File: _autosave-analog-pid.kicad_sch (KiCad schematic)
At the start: 24 parts, among them J1 Conn_01x06_Socket, U1 MCP6004, U2 Opamp_Dual, U3 MCP6004

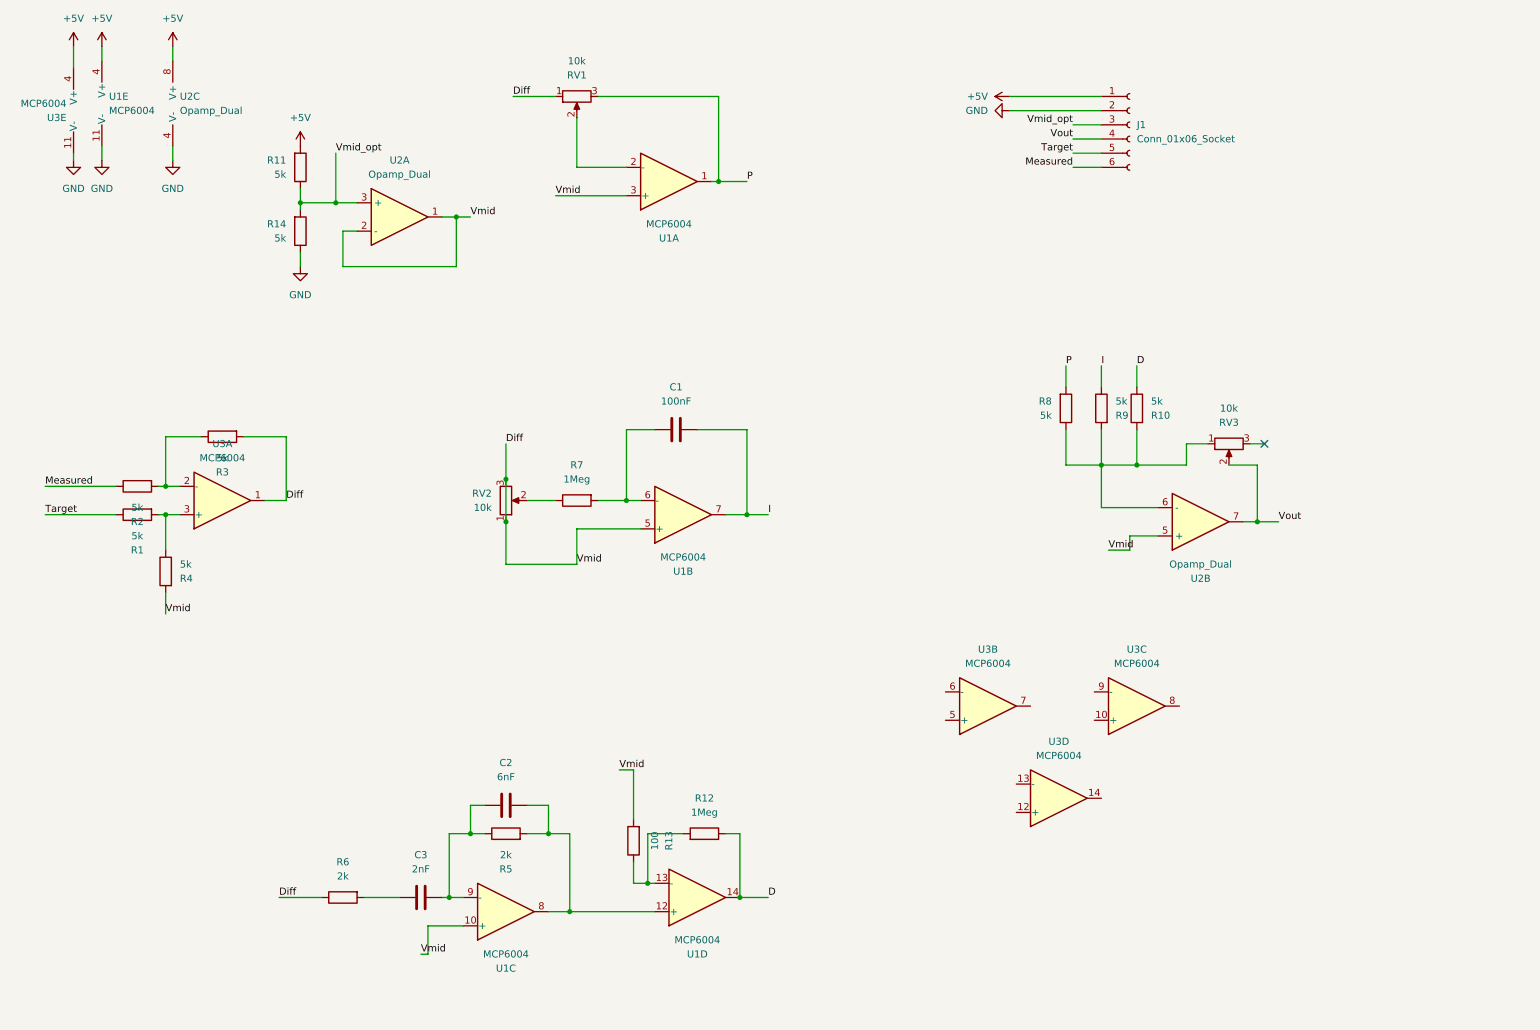
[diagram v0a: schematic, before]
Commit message: second commit before i add even  more fking stuff
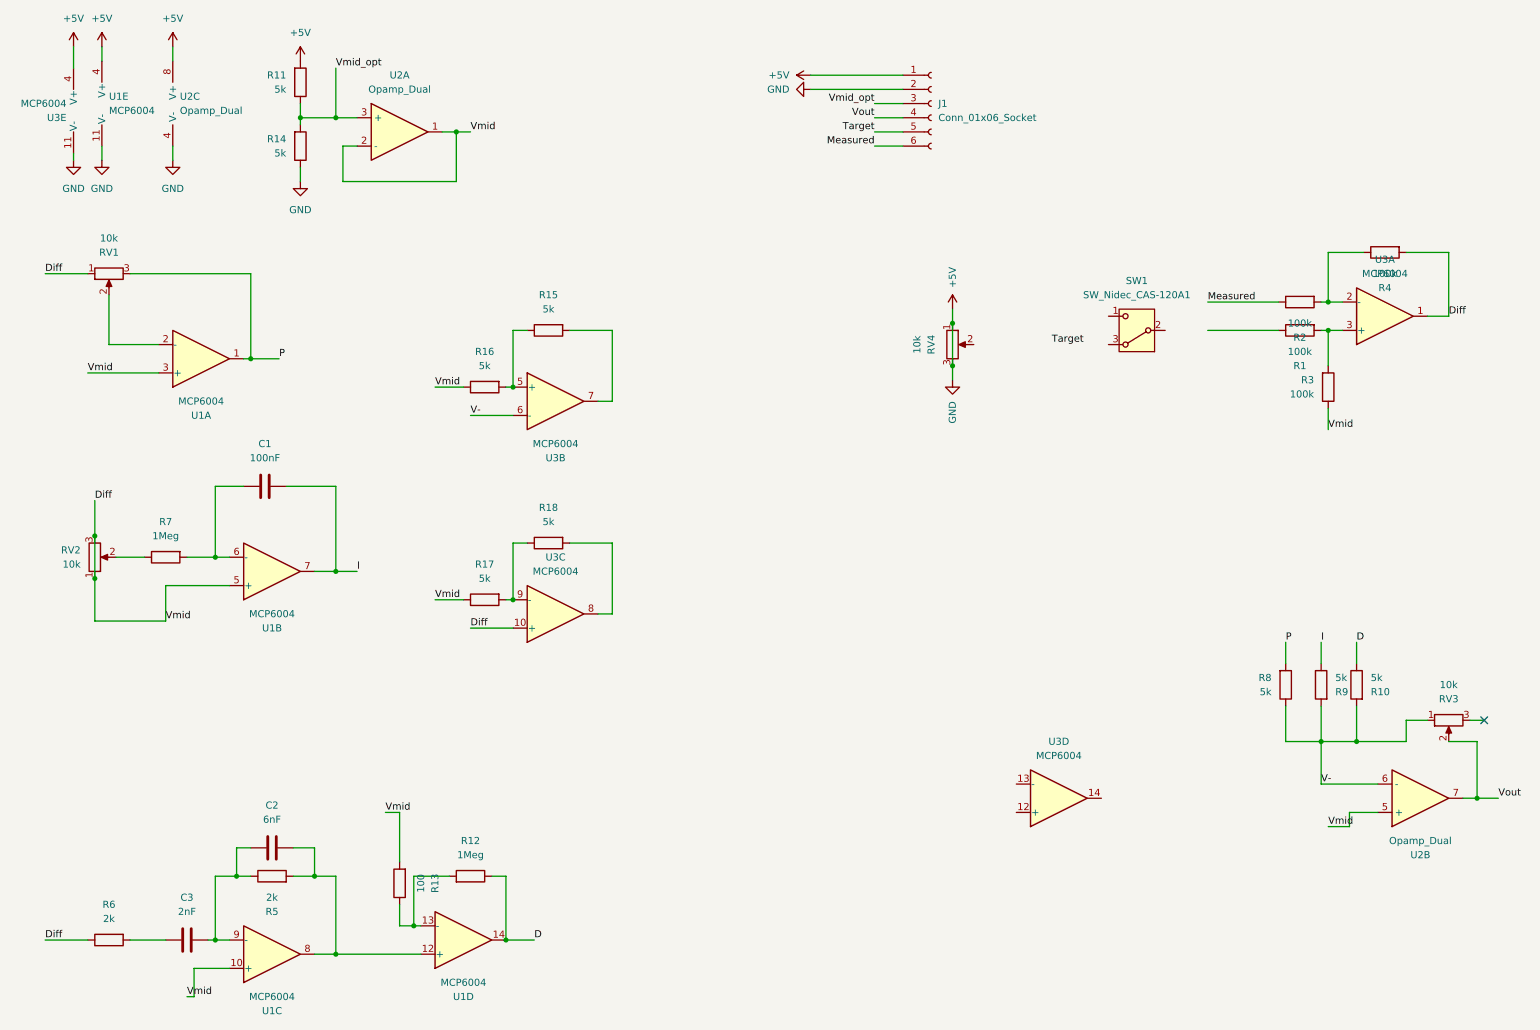
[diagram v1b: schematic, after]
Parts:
- added R15, R16, R17, R18: 5k, symbol Device:R
- added RV4: 10k, symbol Device:R_Potentiometer
- added SW1: SW_Nidec_CAS-120A1, Button_Switch_SMD:Nidec_Copal_CAS-120A, symbol Switch:SW_Nidec_CAS-120A1
- R1, R2, R3, R4: value 5k -> 100k
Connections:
- net GND is gone; now on net +5V: J1.2 (Pin_2), R14.1, U1.11 (V-), U2.4 (V-), U3.11 (V-)
- net +5V: now also RV4.1, RV4.3
- net Diff: now also R3.1, U3.10 (+), R16.1, R17.1; no longer R3.2
- net Target: no longer R1.1
- net at R2.2, U3.2 (-): now also R4.1; no longer R3.1
- net V-: now reaches R10.2, R8.1, R9.2, RV3.1, U2.6 (-)
- net V-: now also U3.6 (-)
- net at R1.2, U3.3 (+): now also R3.2; no longer R4.1
- net at U3.5 (+): now also R15.1, R16.2
- net at U3.7: now also R15.2
- net at U3.8: now also R18.2
- net at U3.9 (-): now also R17.2, R18.1
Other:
- moved on the sheet: C1, C2, C3, J1, R10, R11, R12, R13, R14, R2, R5, R6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
